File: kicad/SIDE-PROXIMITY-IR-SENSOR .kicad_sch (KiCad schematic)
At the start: 10 parts, among them J8 SIDE-PROXI-LEFT, J9 SIDE-PROXI-RIGHT, Q30 RTR030N05HZGTL, Q4 IRLML6344TRPBF

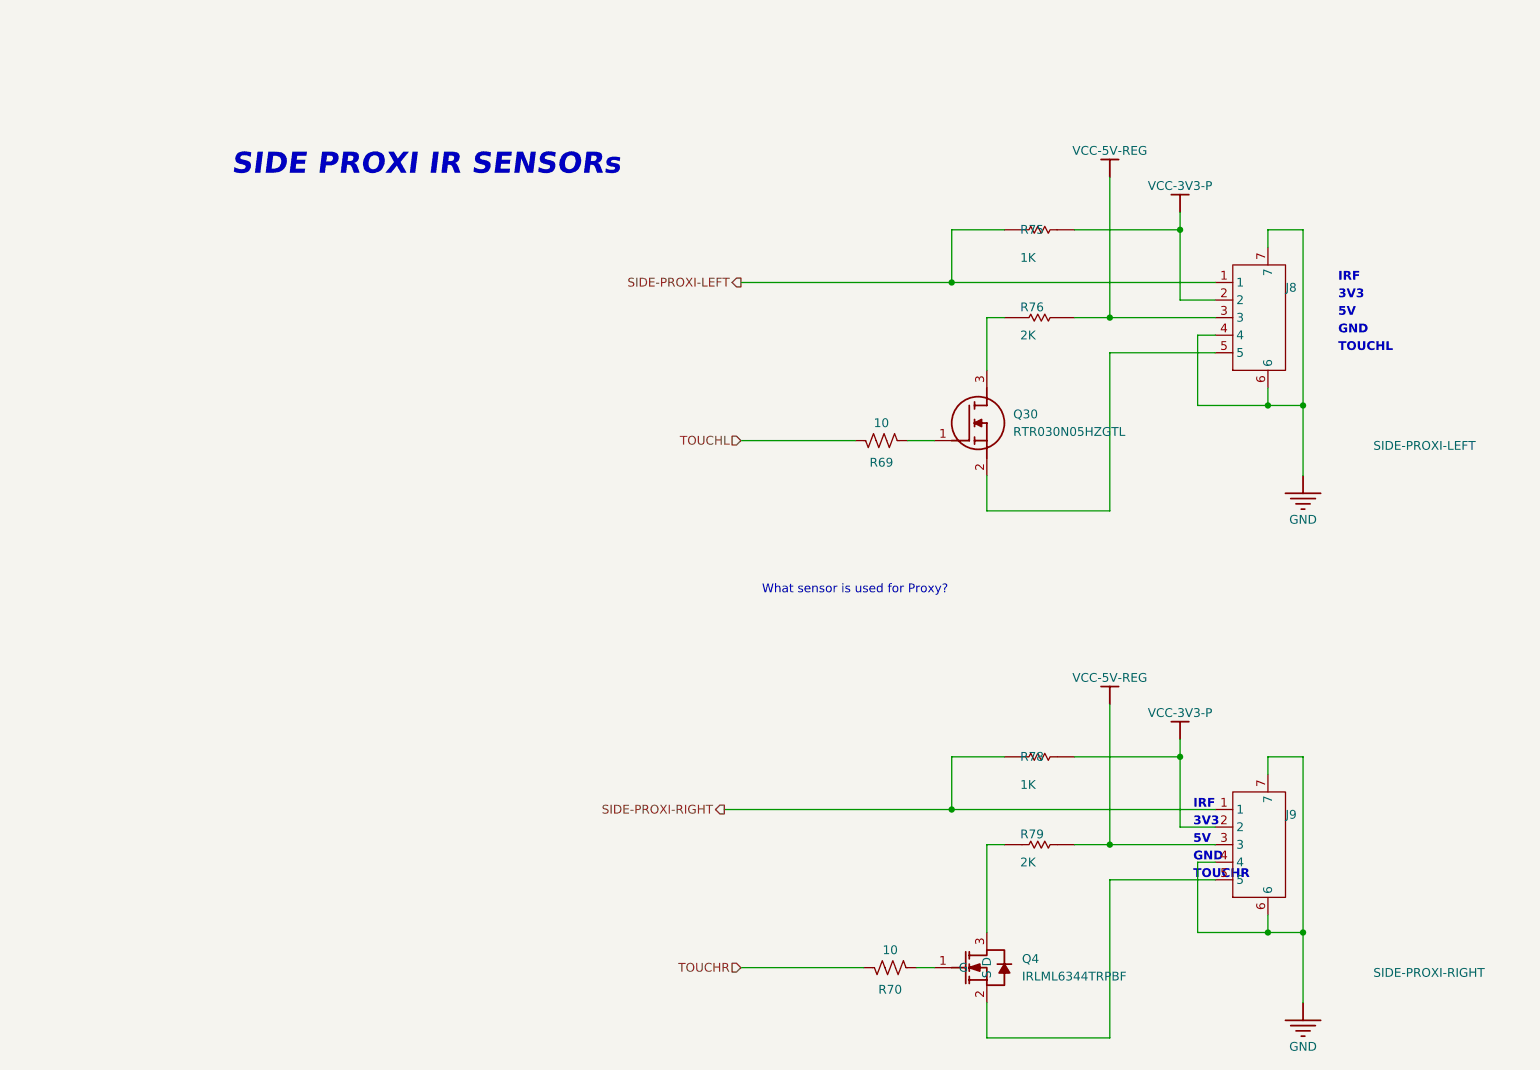
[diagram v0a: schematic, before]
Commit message: External RTC; IR light; side sensors
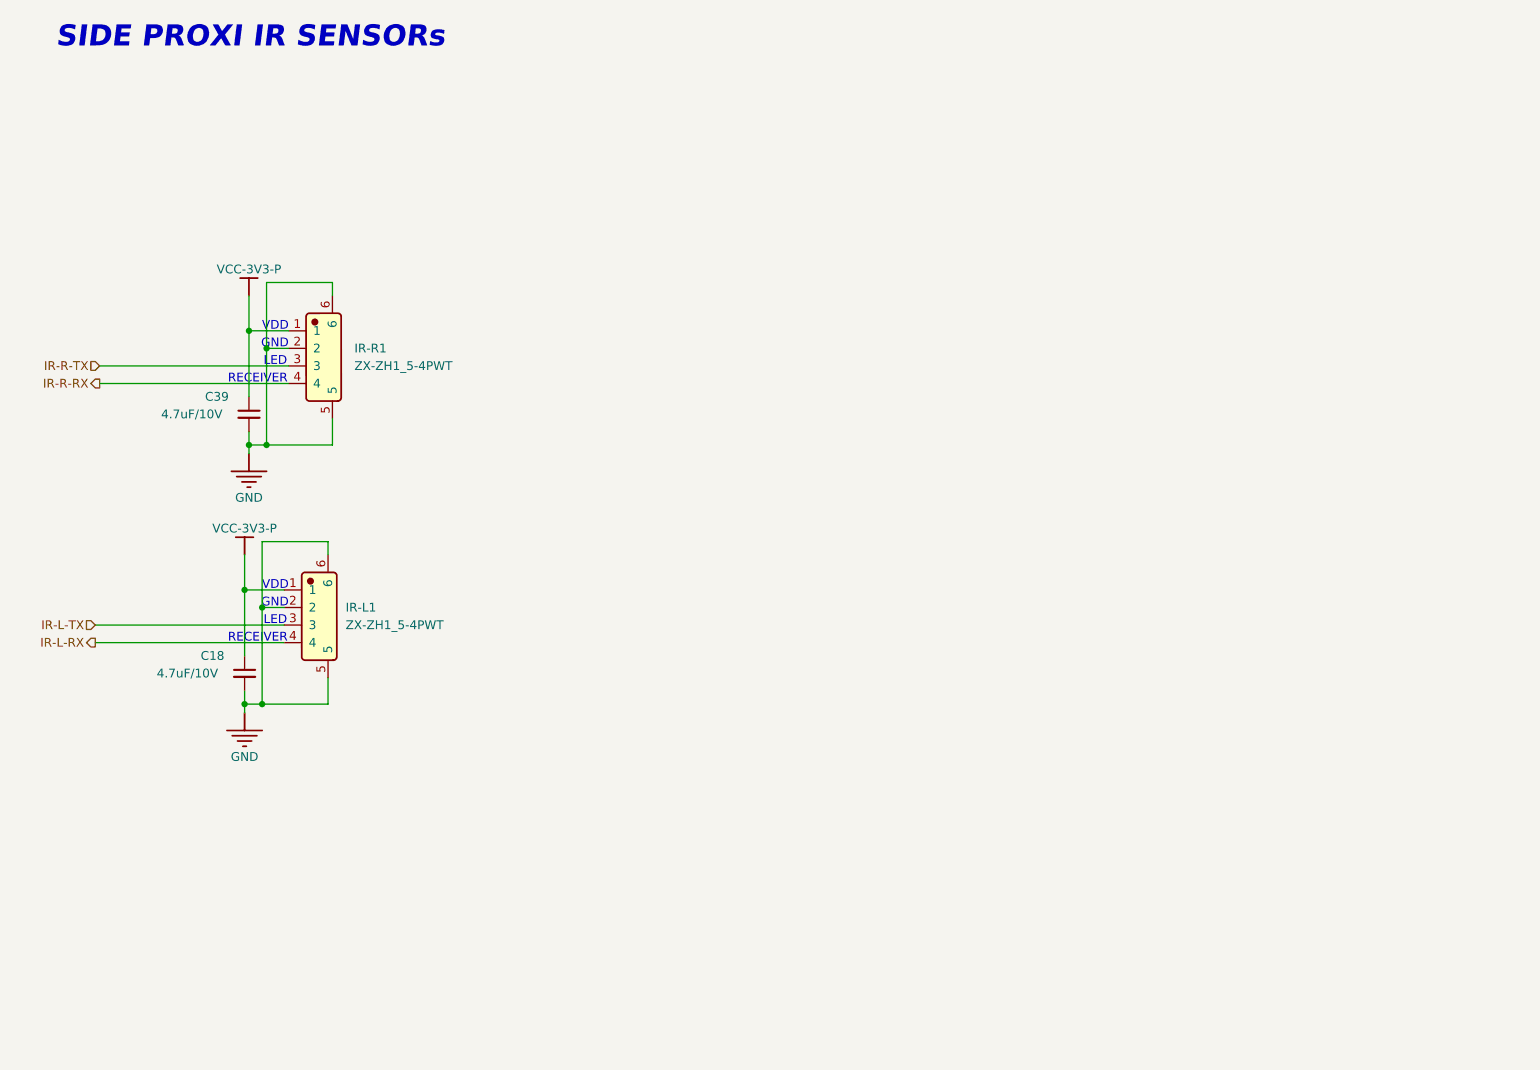
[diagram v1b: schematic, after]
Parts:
- removed J8: SIDE-PROXI-LEFT, oomwoo_altium:CONN-SMD_5P-P1.50_ZX-ZH1.5-5PWT, symbol DesignLibrary:SIDE-PROXI_0_HDRx5_DesignLibrary.SchLib
- removed J9: SIDE-PROXI-RIGHT, oomwoo_altium:CONN-SMD_5P-P1.50_ZX-ZH1.5-5PWT, symbol DesignLibrary:SIDE-PROXI_0_HDRx5_DesignLibrary.SchLib
- removed Q30: RTR030N05HZGTL, LIB_RTR030N05HZGTL:SOT95P280X100-3N, symbol SamacSys_Parts:RTR030N05HZGTL
- removed Q4: IRLML6344TRPBF, JLCImport:IRLML6344TRPBF, symbol JLCImport:IRLML6344TRPBF
- removed R69, R70: 10, Resistor_SMD:R_0603_1608Metric_Pad0.98x0.95mm_HandSolder, symbol Device:R_US
- removed R75, R78: 1K, Resistor_SMD:R_0603_1608Metric, symbol DesignLibrary:SIDE-PROXI_0_Resistor-1_DesignLibrary.SchLib
- removed R76, R79: 2K, Resistor_SMD:R_0603_1608Metric, symbol DesignLibrary:SIDE-PROXI_2_Resistor-1_DesignLibrary.SchLib
- added C18, C39: 4.7uF/10V, symbol Device:C_Small
- added IR-L1, IR-R1: ZX-ZH1_5-4PWT, JLCImport:ZX-ZH1_5-4PWT, symbol JLCImport:ZX-ZH1_5-4PWT
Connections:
- net GND: now also C18.2, C39.2, IR-L1.2, IR-L1.5, IR-L1.6, IR-R1.2, IR-R1.5, IR-R1.6
- net VCC-3V3-P: now also C18.1, C39.1, IR-L1.1, IR-R1.1
- new net IR-L-RX: IR-L1.4
- new net IR-L-TX: IR-L1.3
- new net IR-R-RX: IR-R1.4
- new net IR-R-TX: IR-R1.3
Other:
- note added: "LED"
- note added: "RECEIVER"
- note added: "VDD"
- note removed: "3V3"
- note removed: "5V"
- note removed: "IRF"
- note removed: "TOUCHL"
- note removed: "TOUCHR"
- note removed: "What sensor is used for Proxy?"
